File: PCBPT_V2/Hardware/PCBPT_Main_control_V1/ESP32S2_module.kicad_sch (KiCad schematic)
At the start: 37 parts, among them U7 Wemos/Lolin S2 mini

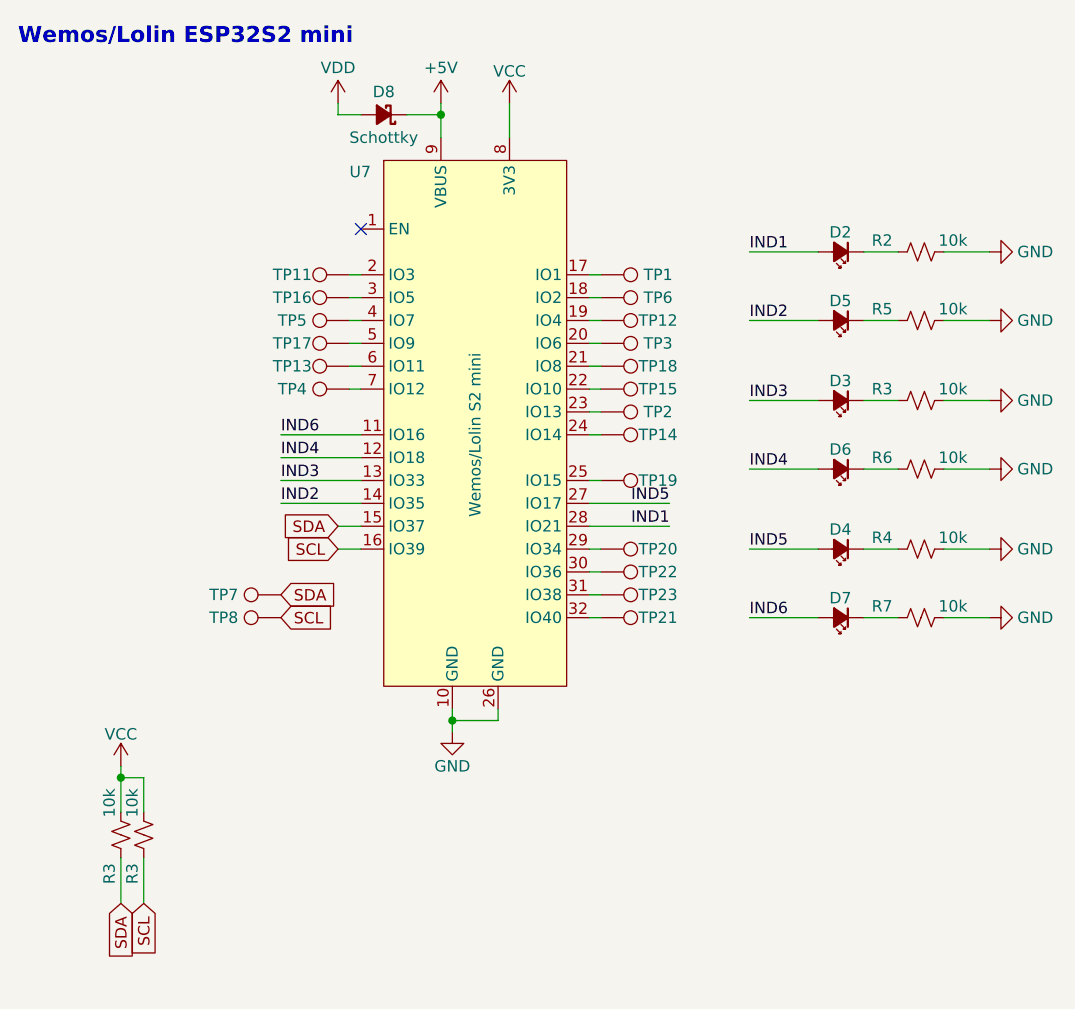
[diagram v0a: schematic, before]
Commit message: udated by FZ
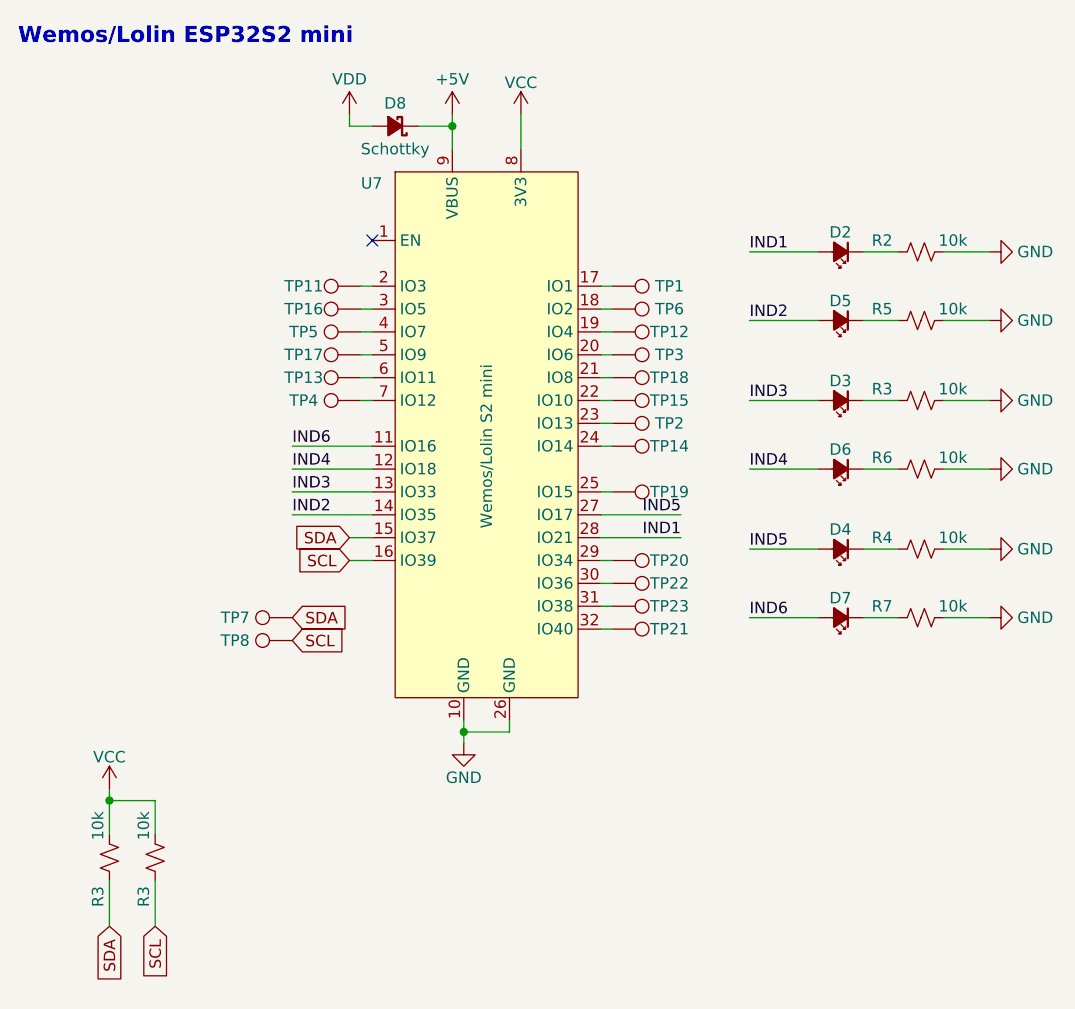
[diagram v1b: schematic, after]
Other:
- moved on the sheet: D8, R3, TP1, TP11, TP12, TP13, TP14, TP15, TP16, TP17, TP18, TP19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
